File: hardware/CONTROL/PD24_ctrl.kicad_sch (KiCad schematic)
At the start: 16 parts, among them J1 Conn_01x12_Socket, J2 Conn_01x08_Socket, SW1 SW_Push, SW2 SW_Push, SW3 SW_Push, U2 STM32G031G8Ux, U5 INA228

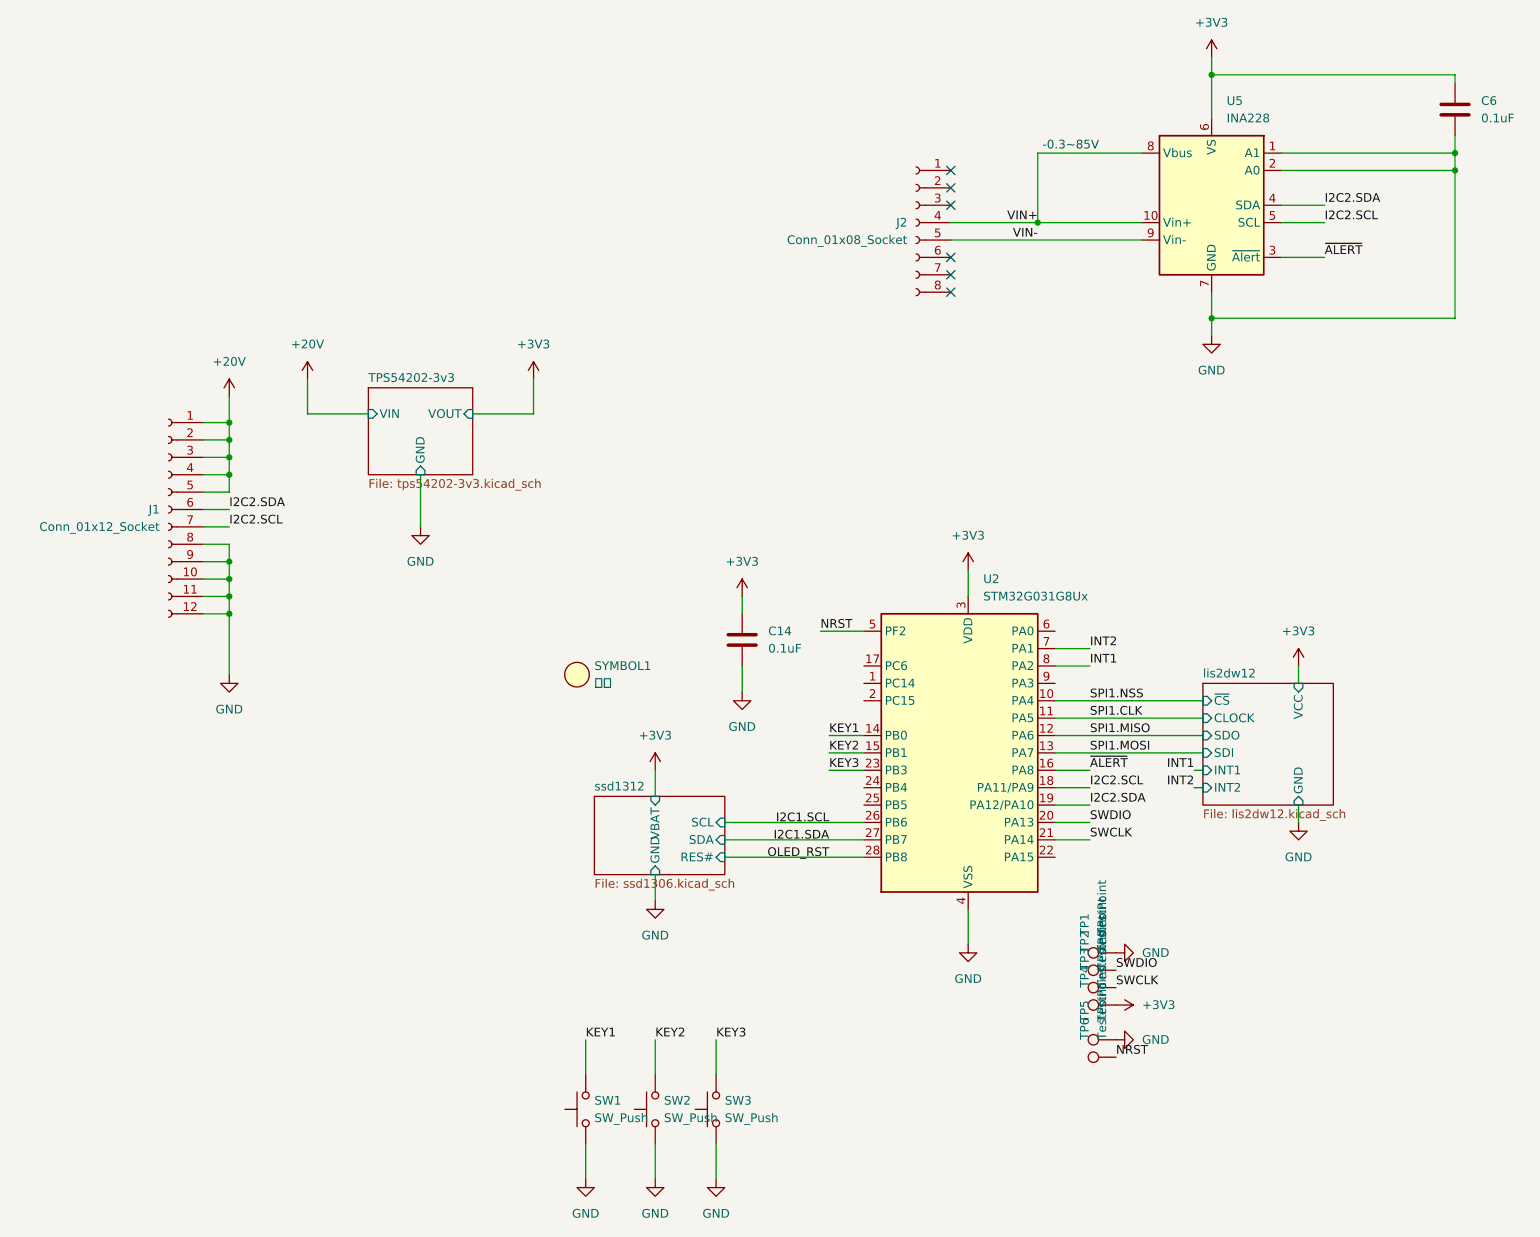
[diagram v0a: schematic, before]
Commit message: 硬件1.0版本更新
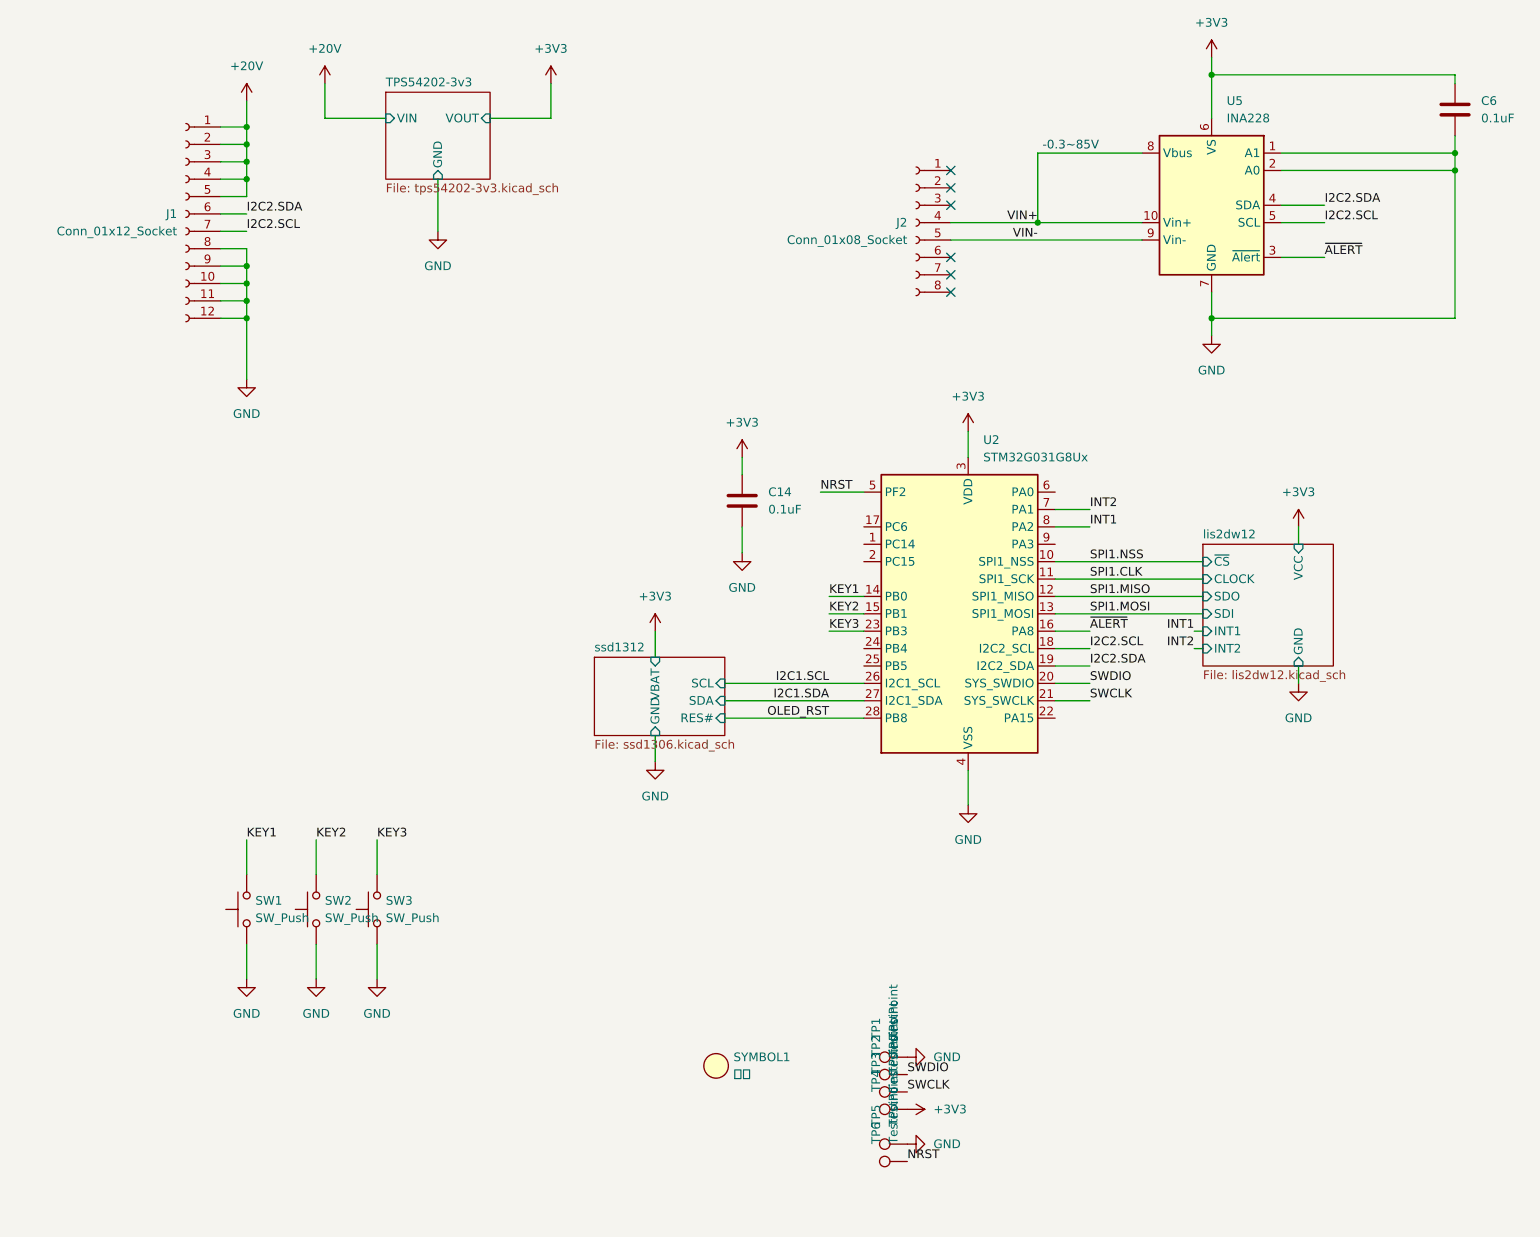
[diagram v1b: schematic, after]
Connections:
- net ssd1312/RES# is gone; now on net OLED_RST: U2.28 (PB8)
- net ssd1312/SCL is gone; now on net I2C1.SCL: U2.26 (PB6)
- net ssd1312/SDA is gone; now on net I2C1.SDA: U2.27 (PB7)
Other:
- moved on the sheet: C14, J1, SW1, SW2, SW3, SYMBOL1, TP1, TP2, TP3, TP4, TP5, TP6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
